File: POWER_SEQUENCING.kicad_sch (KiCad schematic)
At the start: 24 parts, among them U20 74LVC1G08, U21 74LVC1G08, U22 LM397, U23 74LVC1G17, U29 74LVC1G08, U30 74LVC1G08

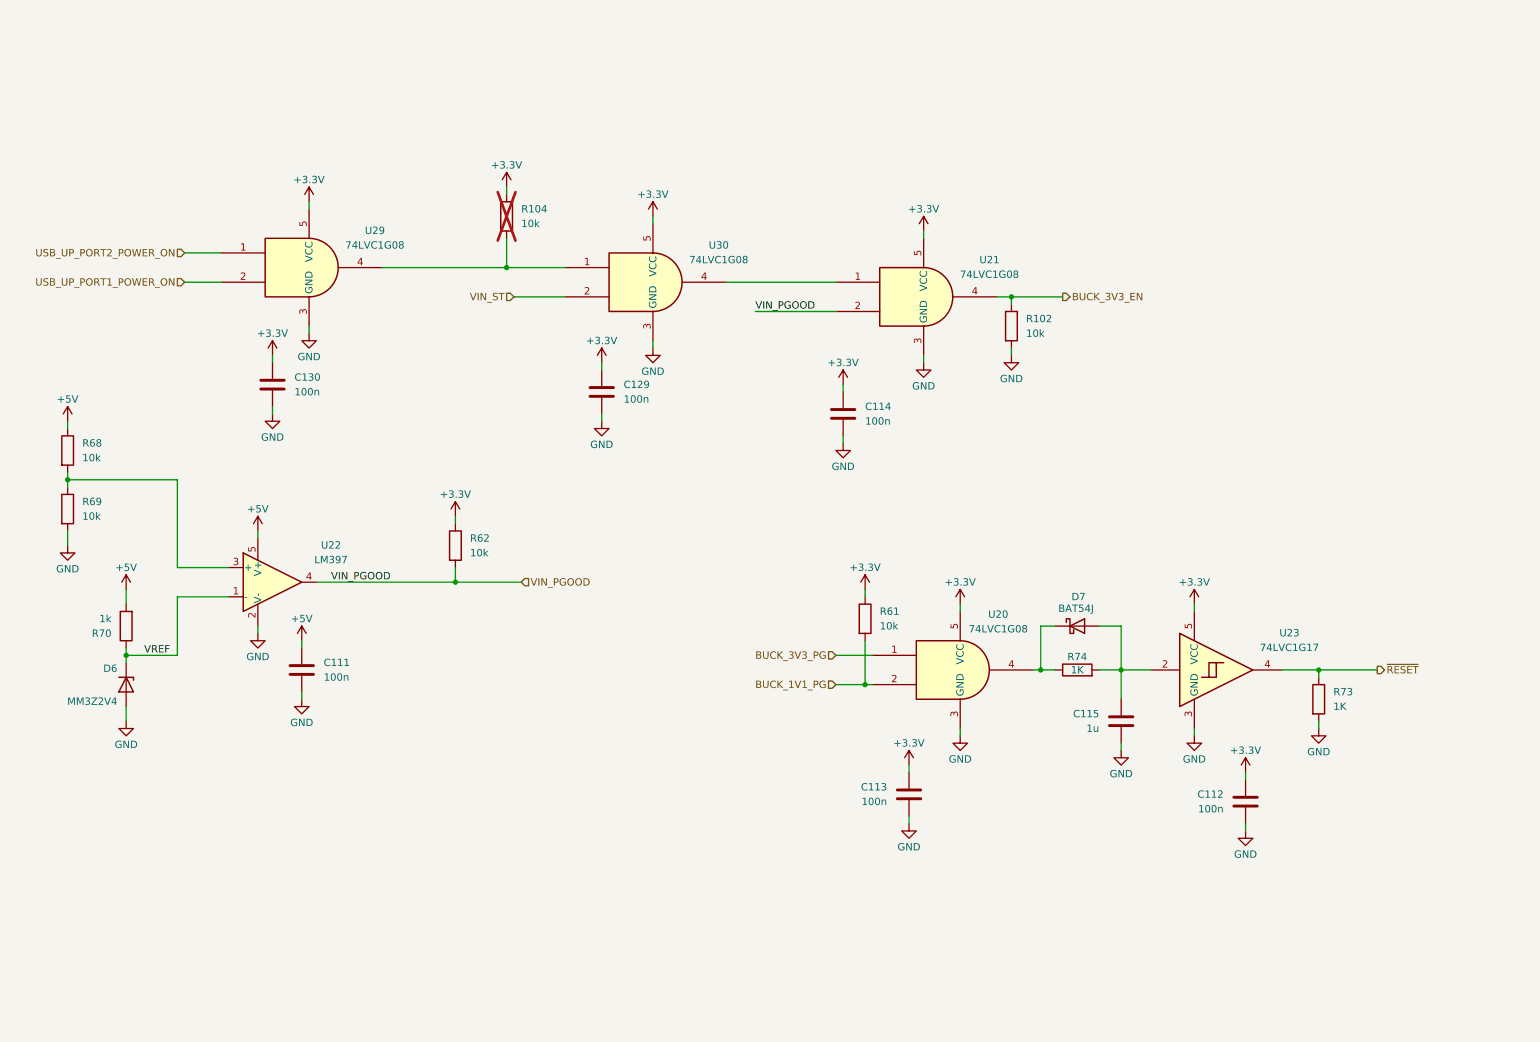
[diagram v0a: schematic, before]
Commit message: Schaltplan erweitert, Kleinzeug
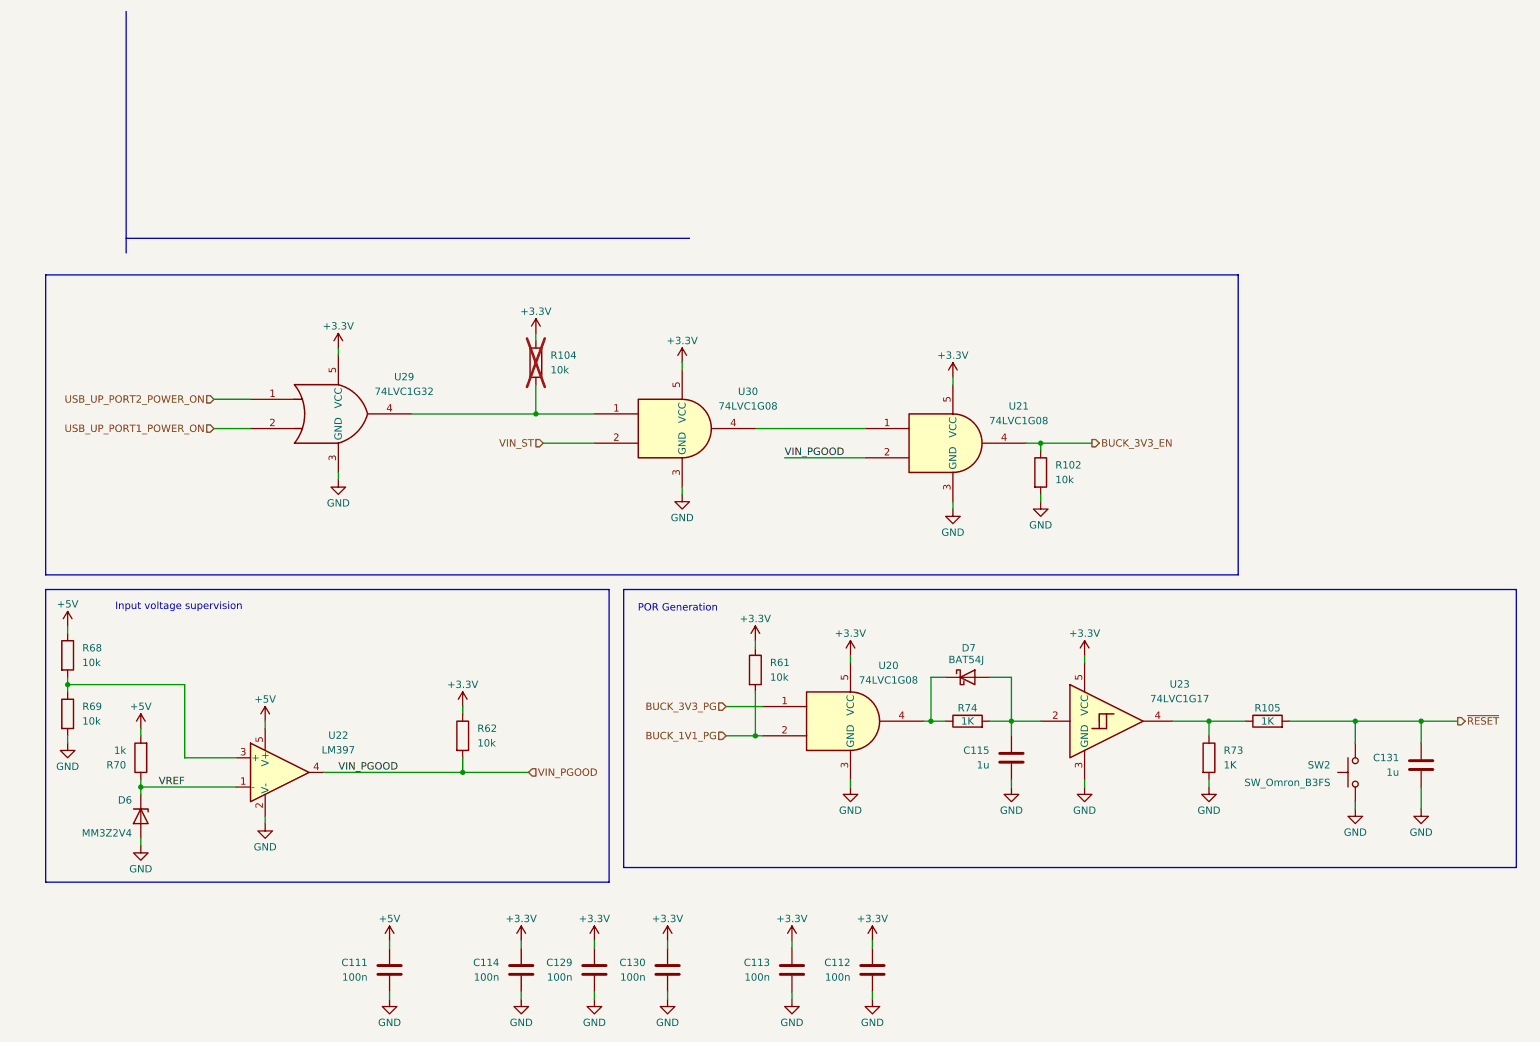
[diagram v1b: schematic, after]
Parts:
- removed U29: 74LVC1G08, Package_TO_SOT_SMD:SOT-23-5, symbol 74xGxx:74LVC1G08
- added C131: 1u, 00_Capacitor:Cap_0402, symbol Device:C
- added R105: 1K, 00_Capacitor:Cap_0402, symbol Device:R
- added SW2: SW_Omron_B3FS, Button_Switch_SMD:SW_SPST_Omron_B3FS-100xP, symbol Switch:SW_Omron_B3FS
- added U29: 74LVC1G32, Package_TO_SOT_SMD:SOT-23-5, symbol 74xGxx:74LVC1G32
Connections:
- net +3.3V: now also U29.5 (VCC)
- net GND: now also C131.2, SW2.1, U29.3 (GND)
- net USB_UP_PORT1_POWER_ON: now also U29.2
- net USB_UP_PORT2_POWER_ON: now also U29.1
- net ~{RESET}: now also C131.1, R105.2, SW2.2; no longer R73.1, U23.4
- net at R104.2, U30.1: now also U29.4
- new net: R105.1, R73.1, U23.4
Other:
- note added: "Input voltage supervision"
- note added: "POR Generation"
- moved on the sheet: C111, C112, C113, C114, C115, C129, C130, D6, D7, R102, R104, R61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
